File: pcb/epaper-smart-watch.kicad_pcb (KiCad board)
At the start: 2 copper layers, 29.2 x 29.2 mm, 66 parts, among them J1 AXT624124, J3 Lithium Battery 3.7V, M1 Motor_DC, P1 USB_C_Plug_USB2.0, Q1 MMBT3904, Q3 Si1308EDL, SW1 BTN, SW2 BTN, SW3 BTN, SW4 BTN, U1 CH340E, U2 STM32WB1MMCH6TR, U3 LSM6DS3

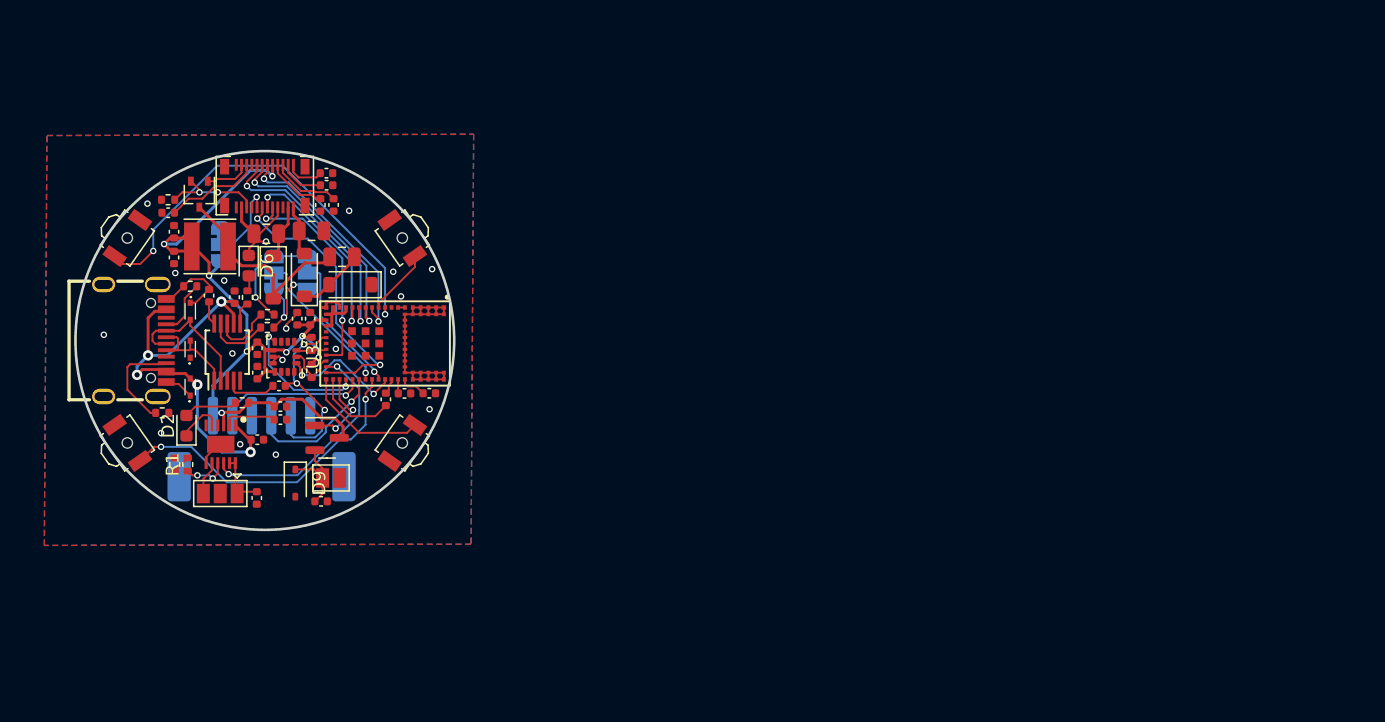
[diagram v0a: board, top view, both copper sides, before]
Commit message: V2 soon...
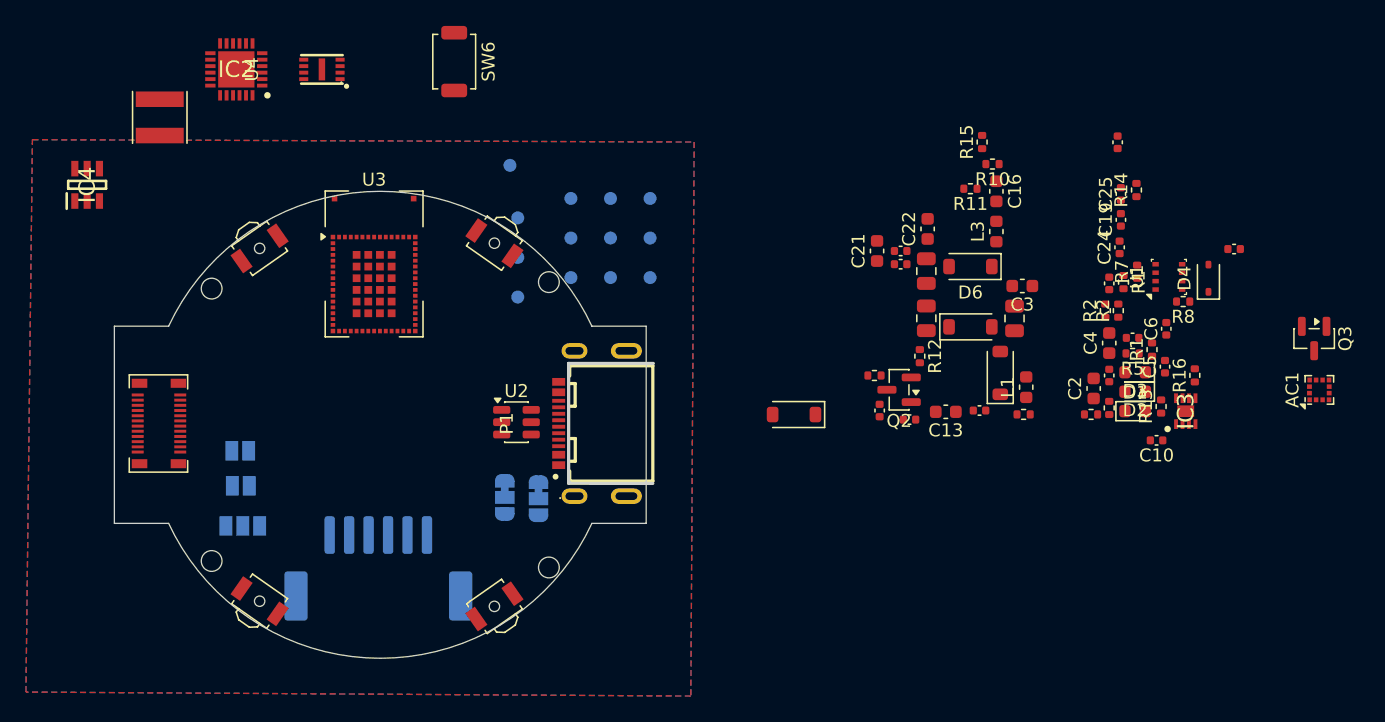
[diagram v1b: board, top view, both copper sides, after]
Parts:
- removed the C20 at (154.6, 100.1)
- removed the C21 at (156.5, 100.1)
- removed the C9 at (147.3, 94.3)
- removed the D1 at (138.0, 93.8)
- removed the D3 at (138.0, 96.7)
- removed the D4 at (138.0, 99.6)
- removed JP3: SolderJumper_3_Bridged12, Jumper:SolderJumper-3_P1.3mm_Bridged12_RoundedPad1.0x1.5mm_NumberLabels
- removed PS1: STNS01PUR, SamacSys:SON45P300X300X80-13N-D
- removed Q1: MMBT3904, Package_TO_SOT_SMD:SOT-23
- removed the R2 at (147.4, 98.3)
- removed the R9 at (136.8, 105.6)
- added AC1: BMA400, Package_LGA:LGA-12_2x2mm_P0.5mm, F.Cu at (225.1, 99.8)
- added BZ1: Buzzer, Jumper:SolderJumper-2_P1.3mm_Open_Pad1.0x1.5mm, B.Cu at (141.9, 107.2)
- added C10: 0.1uF, Capacitor_SMD:C_0402_1005Metric, F.Cu at (212.6, 103.7)
- added C22: 10uF, Capacitor_SMD:C_0603_1608Metric, F.Cu at (194.9, 87.4)
- added C5: 100nF, Capacitor_SMD:C_0402_1005Metric, F.Cu at (213.2, 98.0)
- added C6: 100nF, Capacitor_SMD:C_0402_1005Metric, F.Cu at (213.3, 95.1)
- added D2: LED, LED_SMD:LED_0603_1608Metric, F.Cu at (210.9, 100.0)
- added D6: MBR0530, Diode_SMD:D_SOD-123, F.Cu at (198.2, 90.3)
- added IC2: NPM1100-QDAA-R7, SamasSys:QFN50P400X400X90-25N-D, F.Cu at (141.6, 75.1)
- added IC3: MAX17048G+T10, SamasSys:SON50P200X200X80-9N-D, F.Cu at (214.8, 101.5)
- added IC4: AP3032, SamasSys:SOT95P280X145-6N, F.Cu at (130.1, 84.0)
- added J10: ~, TestPoint:TestPoint_Pad_D1.0mm, B.Cu at (170.4, 85.0)
- added J11: ~, TestPoint:TestPoint_Pad_D1.0mm, B.Cu at (170.4, 88.1)
- added J12: ~, TestPoint:TestPoint_Pad_D1.0mm, B.Cu at (170.4, 91.2)
- added J13: ~, TestPoint:TestPoint_Pad_D1.0mm, B.Cu at (173.5, 85.0)
- added J14: ~, TestPoint:TestPoint_Pad_D1.0mm, B.Cu at (173.5, 88.1)
- added J15: ~, TestPoint:TestPoint_Pad_D1.0mm, B.Cu at (173.5, 91.2)
- added J16: Touch3, TestPoint:TestPoint_Pad_D1.0mm, B.Cu at (163.3, 86.5)
- added J17: Touch2, TestPoint:TestPoint_Pad_D1.0mm, B.Cu at (163.3, 89.6)
- added J18: Touch1, TestPoint:TestPoint_Pad_D1.0mm, B.Cu at (163.3, 92.7)
- added J4: ~, TestPoint:TestPoint_Pad_D1.0mm, B.Cu at (162.7, 82.5)
- added J7: ~, TestPoint:TestPoint_Pad_D1.0mm, B.Cu at (167.4, 85.0)
- added J8: ~, TestPoint:TestPoint_Pad_D1.0mm, B.Cu at (167.4, 88.1)
- added J9: ~, TestPoint:TestPoint_Pad_D1.0mm, B.Cu at (167.4, 91.2)
- added L1: 2.2uH, Inductor_SMD:L_0603_1608Metric, F.Cu at (202.5, 99.6)
- added L3: 6.8uH, Inductor_SMD:L_0603_1608Metric, F.Cu at (200.2, 87.6)
- added Q3: AO3400A, Package_TO_SOT_SMD:SOT-23, F.Cu at (224.7, 95.8)
- added R1: 10k, Resistor_SMD:R_0402_1005Metric, F.Cu at (212.2, 96.7)
- added R1: 10k, Resistor_SMD:R_0402_1005Metric, F.Cu at (210.0, 91.5)
- added R10: 750k, Resistor_SMD:R_0402_1005Metric, F.Cu at (199.9, 82.4)
- added R11: 100k, Resistor_SMD:R_0402_1005Metric, F.Cu at (198.2, 84.3)
- added R13: 1k, Resistor_SMD:R_0402_1005Metric, F.Cu at (212.9, 101.1)
- added R2: 10k, Resistor_SMD:R_0402_1005Metric, F.Cu at (208.6, 93.7)
- added R2: 10k, Resistor_SMD:R_0402_1005Metric, F.Cu at (209.6, 93.7)
- added R5: 8.2k, Resistor_SMD:R_0402_1005Metric, F.Cu at (210.7, 97.0)
- added R8: 100k, Resistor_SMD:R_0402_1005Metric, F.Cu at (214.6, 93.0)
- added SW6: SW_Push, Button_Switch_SMD:SW_SPST_TS-1088-xR020, F.Cu at (158.4, 74.5)
- added U4: XT25F32FDTIGT, ProjectLibrary:DFN-8_L3.0-W2.0-P0.50-BL-EP_XT25XXX, F.Cu at (148.2, 75.1)
- C11: renamed from C13; value 2.2uF -> 100nF
- C13: renamed from C1; footprint Capacitor_SMD:C_0402_1005Metric -> Capacitor_SMD:C_0603_1608Metric
- C16: value 4.7uF -> 1uF; footprint Capacitor_SMD:C_0402_1005Metric -> Capacitor_SMD:C_0603_1608Metric
- C19: value 2.7pF -> 1uF/16V
- C2: renamed from C17; value 0.1uF -> 10uF; footprint Capacitor_SMD:C_0402_1005Metric -> Capacitor_SMD:C_0603_1608Metric
- C21: renamed from C4; footprint Capacitor_SMD:C_0402_1005Metric -> Capacitor_SMD:C_0603_1608Metric
- C22: value 2.2uF -> 3.3pF
- C24, C25: value 0.1uF -> 100nF
- C3: renamed from C18; footprint Capacitor_SMD:C_0402_1005Metric -> Capacitor_SMD:C_0603_1608Metric
- C4: renamed from C15; value 0.1uF -> 10uF; footprint Capacitor_SMD:C_0402_1005Metric -> Capacitor_SMD:C_0603_1608Metric
- C7: renamed from C14; value 1uF -> 2.2uF
- C8: renamed from C12; value 4.7uF -> 1uF
- J5: renamed from J3; moved to B.Cu
- J6: renamed from J1; footprint FPC:AXT624124 -> ProjectLibrary:AXT624124
- M1: moved to B.Cu
- P1: footprint USBC:USB-C-SMD_KH-TYPE-C-16P -> ProjectLibrary:USB-C-SMD_TYPE-C-16P-CB0.8-073
- Q2: renamed from Q3; footprint Package_TO_SOT_SMD:SOT-323_SC-70 -> Package_TO_SOT_SMD:SOT-23
- R12: renamed from R1; value 2k -> 100k
- R14: value 1k -> 100k
- R15: value 1k -> 10
- R16: value 1k -> 10k
- R6: renamed from R5; value 600 -> 1k
- R7: value 10K -> 100
- U1: value CH340E -> BME280; footprint Package_SO:MSOP-10_3x3mm_P0.5mm -> Package_LGA:Bosch_LGA-8_2.5x2.5mm_P0.65mm_ClockwisePinNumbering
- U2: value STM32WB1MMCH6TR -> USBLC6-2SC6; footprint EasyEda2Kicad:LGA-77_L10.0-W6.5-STM32WB1MMCH6TR -> Package_TO_SOT_SMD:SOT-23-6
- U3: value LSM6DS3 -> STM32WB5MMG; footprint Package_LGA:LGA-14_3x2.5mm_P0.5mm_LayoutBorder3x4y -> RF_Module:ST-SiP-LGA-86-11x7.3mm
- moved D3 73.3 mm to (210.9, 98.5), turned to 180 degrees
- moved C9 73.0 mm to (218.5, 89.0)
- moved U1 72.8 mm to (213.5, 91.1)
- moved D4 72.1 mm to (216.6, 91.2), turned to 90 degrees
- moved R3 71.6 mm to (207.5, 101.7)
- moved R16 71.6 mm to (215.5, 98.7), turned to 90 degrees
- moved D1 69.3 mm to (210.9, 101.5), turned to 0 degrees
- moved R14 69.0 mm to (211.0, 84.4)
- moved C2 68.6 mm to (207.7, 99.7)
- moved C22 68.0 mm to (209.6, 80.7), turned to 90 degrees
- moved C11 67.9 mm to (210.7, 95.8), turned to 180 degrees
- moved C8 67.8 mm to (208.9, 91.6), turned to 90 degrees
- moved C25 67.6 mm to (209.8, 84.7), turned to 90 degrees
- moved C4 67.5 mm to (208.9, 96.2)
- moved C24 67.2 mm to (209.7, 88.8)
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- renumbered C2 to C12, C8 to C14, C3 to C15, C11 to C17, C7 to C18, C6 to C19, C5 to C20, C10 to C23, C23 to C9, D6 to D1, D2 to D3, D9 to D4, D7 to D5, D5 to D7, L1 to L2, R6 to R9, SW1 to SW2, SW2 to SW3, SW3 to SW4, SW4 to SW5
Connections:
- net /RESR renamed /EPD_RESR
- net /VCOM renamed /EPD_VCOM
- net /VGH renamed /EPD_VGH
- net /VGL renamed /EPD_VGL
- C11 pad 1: /VBUS -> +3V0
- C12 pad 1: /EPD_VDD -> +3V0
- C13 pad 1: /EPD_VDD -> +3V0
- C16 pad 1: /EPD_VDD -> /EPD_LIGHT_PWR_POS
- C16 pad 2: GND -> /EPD_LIGHT_PWR_NEG
- C19 pad 1: Net-(U2-PB1) -> Net-(J6-Pin_5)
- C19 pad 1: Net-(J1-Pin_5) -> Net-(J6-Pin_5)
- C2 pad 1: Net-(U1-V3) -> +3V0
- C24 pad 1: /EPD_VDD -> GND
- C24 pad 2: GND -> /NRST
- C25 pad 1: /EPD_VDD -> GND
- C25 pad 2: GND -> Net-(U3-PC13)
- C3 pad 1: Net-(U1-~{RTS}) -> Net-(IC2-DEC)
- C3 pad 2: /NRST -> GND
- C4 pad 1: /VBUS -> /VSYS
- C7 pad 1: /EPD_VDD -> +5V
- C9 pad 1: Net-(D9-K) -> +3V0
- C9 pad 2: GND -> Net-(D4-A)
- D1 pad 1: GND -> Net-(D1-K)
- D1 pad 2: Net-(D6-A) -> /VSYS
- D3 pad 1: /CHG -> GND
- D4 pad 1: Net-(D9-K) -> +3V0
- D4 pad 2: GND -> Net-(D4-A)
- J5 pad 2: GND -> Net-(J5-Pin_2)
- J5 pad 3: Net-(J3-Pin_3) -> GND
- J6 pad 12: /CSB -> /EPD_CSB
- J6 pad 13: /DC -> /EPD_DC
- J6 pad 14: /RST_N -> /EPD_RST_N
- J6 pad 15: /BUSY -> /EPD_BUSY
- J6 pad 16: Net-(J1-Pin_16) -> Net-(J6-Pin_16)
- J6 pad 21: /GDR -> /EPD_GDR
- J6 pad 23: /FL+ -> /EPD_LIGHT_PWR_POS
- J6 pad 24: /FL- -> /EPD_LIGHT_PWR_NEG
- J6 pad 5: Net-(J1-Pin_5) -> Net-(J6-Pin_5)
- J6 pad 9: /EPD_VDD -> +3V0
- JP1 pad 1: Net-(JP1-A) -> Net-(J6-Pin_16)
- JP1 pad 2: /TXD -> GND
- JP1 pad 3: Net-(JP1-B) -> +3V0
- JP2 pad 1: Net-(JP1-B) -> Net-(JP2-A)
- JP2 pad 2: /RXD -> Net-(IC2-NTC)
- JP2 pad 3: Net-(JP1-A) -> Net-(J5-Pin_2)
- L2 pad 1: /EPD_VDD -> +3V0
- M1 pad 1: Net-(D9-K) -> +3V0
- M1 pad 2: GND -> Net-(D4-A)
- P1 pad A6: /D+ -> Net-(P1-D+-PadA6)
- P1 pad A7: /D- -> Net-(P1-D--PadA7)
- P1 pad A8: unconnected-(P1-SBU1-PadA8) -> (no net)
- P1 pad B6: /D+ -> Net-(P1-D+-PadA6)
- P1 pad B7: /D- -> Net-(P1-D--PadA7)
- P1 pad B8: unconnected-(P1-SBU2-PadB8) -> (no net)
- Q2 pad 1: /GDR -> /EPD_GDR
- R12 pad 1: Net-(PS1-ISET) -> GND
- R12 pad 2: Net-(R1-Pad2) -> /EPD_GDR
- R14 pad 1: Net-(U1-TNOW) -> +3V0
- R14 pad 2: Net-(D6-A) -> /FLASH_CS
- R15 pad 1: Net-(U1-TXD) -> GND
- R15 pad 2: Net-(JP1-A) -> /EPD_LIGHT_PWR_NEG
- R16 pad 1: Net-(U1-RXD) -> Net-(JP2-A)
- R16 pad 2: Net-(JP1-B) -> GND
- R6 pad 1: /EPD_VDD -> +5V
- R7 pad 1: /EPD_VDD -> Net-(Q3-G)
- R7 pad 2: /Accel_SDA -> /VIB
- SWD1 pad 6: /EPD_VDD -> +3V0
- U1 pad 1: /D+ -> GND
- U1 pad 2: /D- -> Net-(U1-CSB)
- U1 pad 3: GND -> /ACCL_SDA
- U1 pad 4: Net-(U1-~{RTS}) -> /ACCL_SCL
- U1 pad 5: unconnected-(U1-~{CTS}-Pad5) -> GND
- U1 pad 6: Net-(U1-TNOW) -> +3V0
- U1 pad 7: /VBUS -> GND
- U1 pad 8: Net-(U1-TXD) -> +3V0
- U2 pad 1: GND -> Net-(P1-D--PadA7)
- U2 pad 3: GND -> Net-(P1-D+-PadA6)
- U2 pad 4: GND -> /D+
- U2 pad 5: GND -> +5V
- U2 pad 6: Net-(U2-ANT_IN) -> /D-
- U3 pad 1: unconnected-(U3-SDO/SA0-Pad1) -> /EPD_BUSY
- U3 pad 10: unconnected-(U3-NC-Pad10) -> /NRST
- U3 pad 11: unconnected-(U3-NC-Pad11) -> /ACCL_SDA
- U3 pad 12: /Accel_CS -> /ACCL_INT1
- U3 pad 13: /Accel_SCL -> Net-(U3-PH3-BOOT0)
- U3 pad 14: /Accel_SDA -> /ACCL_SCL
- U3 pad 4: /Accel_INT1 -> +3V0
- U3 pad 5: /EPD_VDD -> GND
- U3 pad 6: GND -> +3V0
- U3 pad 7: GND -> unconnected-(U3-PC3-Pad7)
- U3 pad 8: /EPD_VDD -> unconnected-(U3-PC2-Pad8)
- U3 pad 9: unconnected-(U3-INT2-Pad9) -> /ACCL_INT2
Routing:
- net /EPD_VDD: track 71.7 -> 0.00 mm, vias 8 -> 0
- net GND: track 54.7 -> 0.00 mm, vias 17 -> 0
- net /VBUS: track 34.2 -> 0.00 mm, vias 5 -> 0
- net /BTN_1: track 32.7 -> 0.00 mm, vias 2 -> 0
- net /BTN_4: track 24.7 -> 0.00 mm, vias 2 -> 0
- net /RST_N: track 22.1 -> 0.00 mm, vias 2 -> 0
- net /BUSY: track 18.6 -> 0.00 mm, vias 2 -> 0
- net /DC: track 18.4 -> 0.00 mm, vias 2 -> 0
- net /BATMS: track 18.3 -> 0.00 mm, vias 2 -> 0
- net /EPD_SPICL: track 18.1 -> 0.00 mm, vias 2 -> 0
- net /EPD_MOSI: track 17.0 -> 0.00 mm, vias 2 -> 0
- net /CSB: track 15.1 -> 0.00 mm, vias 2 -> 0
- net Net-(D5-A): track 15.0 -> 0.00 mm
- net /NRST: track 14.9 -> 0.00 mm, vias 3 -> 0
- net /RXD: track 11.7 -> 0.00 mm, vias 1 -> 0
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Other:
- board size 29.2 x 29.2 mm -> 41 x 36 mm
- copper layers 2 -> 4
